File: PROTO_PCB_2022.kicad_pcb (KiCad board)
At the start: 2 copper layers, 92.1 x 40.6 mm, 22 parts, among them J1 HORN_EN1, J10 ECU_KILL_2, J11 ECU_KILL_3, J12 12V_EXTRA, J2 BRAKELIGHTS_EN1, J3 BRAKELIGHTS_CONN, J4 STARTER_MOTOR_EN, J5 VESC_EN_SIGNAL, J6 HORN_CONN, J7 12V_BATT1, J8 ECU_POWER_DIST, J9 ECU_KILL_1, Q1 , Q2 , U1 

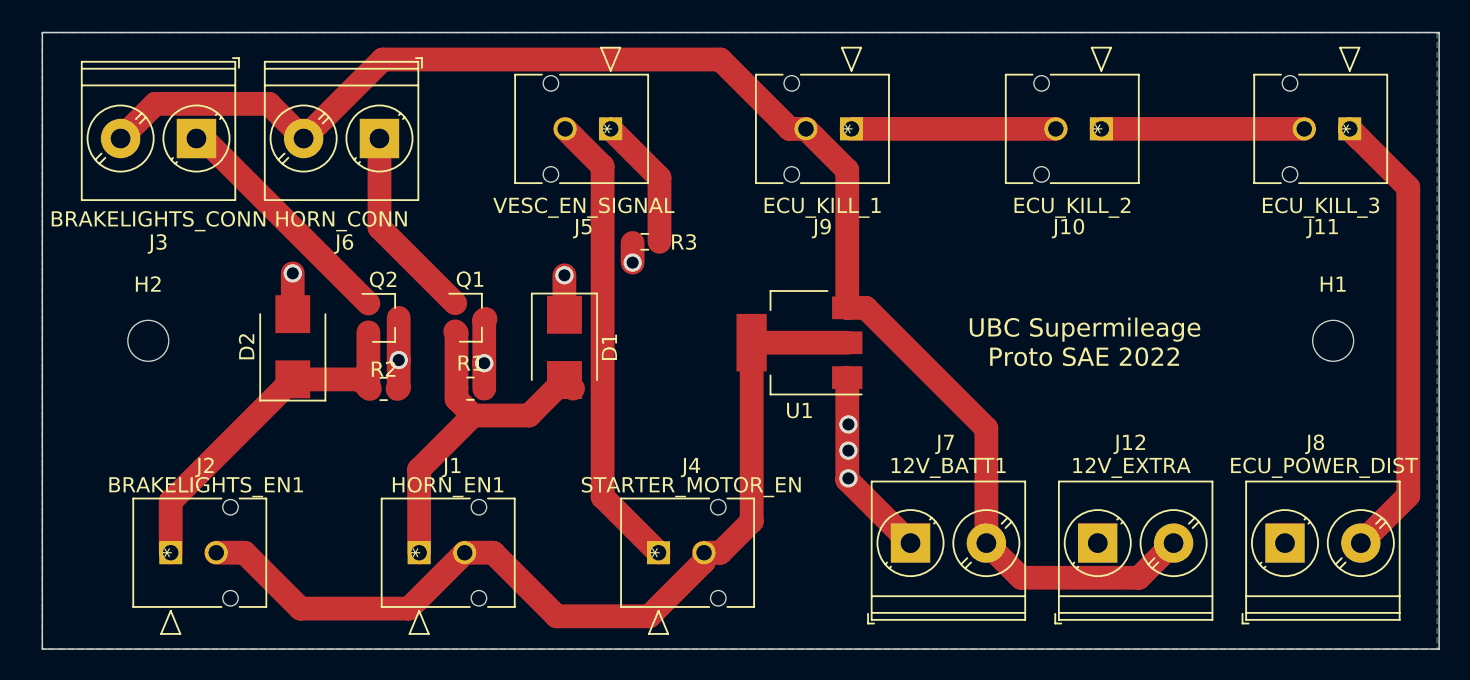
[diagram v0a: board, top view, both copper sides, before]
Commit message: almost final version
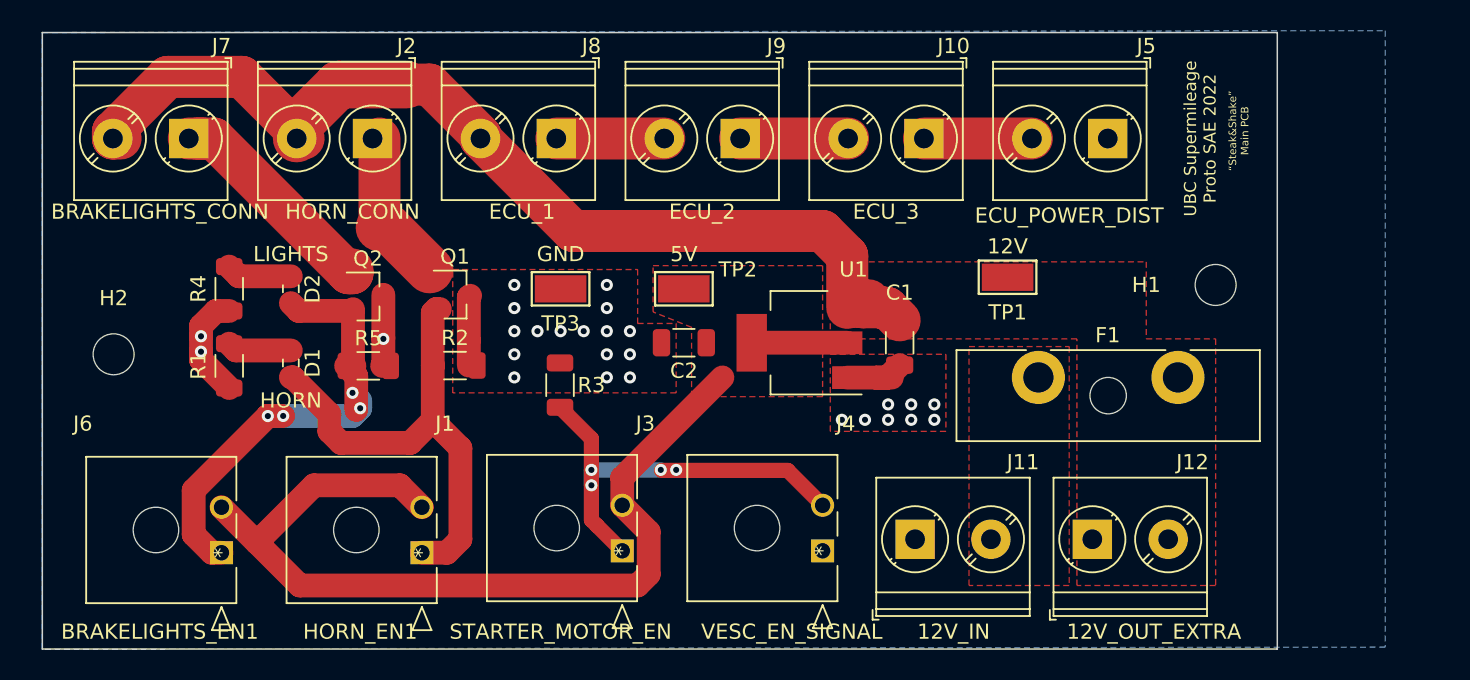
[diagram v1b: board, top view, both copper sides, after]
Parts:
- removed the J11 at (156.7, 84.5)
- added C1: 1u, Capacitor_SMD:C_1206_3216Metric, F.Cu at (127.0, 98.6)
- added C2: 4.7u, Capacitor_SMD:C_1206_3216Metric, F.Cu at (112.8, 98.6)
- added F1: Fuse, Fuse:Fuseholder_Blade_ATO_Littelfuse_Pudenz_2_Pin, F.Cu at (136.1, 100.8)
- added J8: ECU_1, TerminalBlock_Phoenix:TerminalBlock_Phoenix_PT-1,5-2-5.0-H_1x02_P5.00mm_Horizontal, F.Cu at (104.4, 85.1)
- added R1: 4.7k, Resistor_SMD:R_1206_3216Metric, F.Cu at (82.8, 100.1)
- added R4: 4.7k, Resistor_SMD:R_1206_3216Metric, F.Cu at (82.8, 95.0)
- added TP1: TestPoint, TestPoint:TestPoint_Keystone_5015_Micro-Minature, F.Cu at (134.1, 94.2)
- added TP2: TestPoint, TestPoint:TestPoint_Keystone_5015_Micro-Minature, F.Cu at (112.8, 95.0)
- added TP3: TestPoint, TestPoint:TestPoint_Keystone_5015_Micro-Minature, F.Cu at (104.6, 95.0)
- D1, D2: value (none) -> LED; footprint Diode_SMD:D_SMB -> Resistor_SMD:R_0603_1608Metric
- J1: footprint Footprint Library:Molex_Proto_Microfit_Footprint -> footprints:436500201
- J10: value ECU_KILL_2 -> ECU_3; footprint Footprint Library:Molex_Proto_Microfit_Footprint -> TerminalBlock_Phoenix:TerminalBlock_Phoenix_PT-1,5-2-5.0-H_1x02_P5.00mm_Horizontal
- J11: renamed from J7; value 12V_BATT1 -> 12V_IN
- J12: value 12V_EXTRA -> 12V_OUT_EXTRA
- J3: renamed from J4; footprint Footprint Library:Molex_Proto_Microfit_Footprint -> footprints:436500201
- J4: renamed from J5; footprint Footprint Library:Molex_Proto_Microfit_Footprint -> footprints:436500201
- J6: renamed from J2; footprint Footprint Library:Molex_Proto_Microfit_Footprint -> footprints:436500201
- J9: value ECU_KILL_1 -> ECU_2; footprint Footprint Library:Molex_Proto_Microfit_Footprint -> TerminalBlock_Phoenix:TerminalBlock_Phoenix_PT-1,5-2-5.0-H_1x02_P5.00mm_Horizontal
- Q1: value (none) -> HORN_MOSFET1
- Q2: value (none) -> BRAKELIGHTS_MOSFET1
- R2: renamed from R1; footprint Resistor_SMD:R_0805_2012Metric -> Resistor_SMD:R_1206_3216Metric
- R3: value (none) -> 10k; footprint Resistor_SMD:R_0603_1608Metric -> Resistor_SMD:R_1206_3216Metric
- R5: renamed from R2; value (none) -> 10k; footprint Resistor_SMD:R_0805_2012Metric -> Resistor_SMD:R_1206_3216Metric
- U1: value (none) -> LD1117S50TR_SOT223
- moved J4 31.1 mm to (121.9, 112.3), turned to 270 degrees
- moved J5 29.1 mm to (140.7, 85.1), turned to 180 degrees
- moved D1 18.1 mm to (86.9, 99.9)
- moved J10 11.7 mm to (128.6, 85.1), turned to 180 degrees
- moved R3 11.0 mm to (104.6, 101.3), turned to 90 degrees
- moved H1 8.58 mm to (147.8, 94.7)
- moved J9 7.37 mm to (116.5, 85.1), turned to 180 degrees
- moved D2 3.82 mm to (86.9, 95.0), turned to 270 degrees
- moved J6 3.35 mm to (82.3, 112.4)
- moved H2 2.45 mm to (75.2, 99.3)
- moved J3 2.40 mm to (108.7, 112.3)
- moved Q1 1.83 mm to (97.7, 95.4)
- moved R2 1.83 mm to (97.7, 100.1)
- moved R5 1.83 mm to (92.0, 100.1)
- moved Q2 1.75 mm to (91.9, 95.5)
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- renumbered J6 to J2, J8 to J5, J3 to J7
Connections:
- D1 pad 1: GND -> Net-(D1-Pad1)
- D2 pad 1: BRAKELIGHTS_EN_5V -> Net-(D2-Pad1)
- D2 pad 2: GND -> BRAKELIGHTS_EN_5V
- J10 pad 1: ECU_KILL_EN_TOGGLESWITCH_2B -> ECU_KILL_EN_TOGGLESWITCH_3B
- J10 pad 2: ECU_KILL_EN_TOGGLESWITCH_1B -> ECU_KILL_EN_TOGGLESWITCH_2B
- J11 pad 2: 12V_FOR_BRAKELIGHTS -> BATT_12V
- J4 pad 1: Net-(J5-Pad1) -> GND
- J9 pad 1: ECU_KILL_EN_TOGGLESWITCH_1B -> ECU_KILL_EN_TOGGLESWITCH_2B
- J9 pad 2: 12V_FOR_BRAKELIGHTS -> ECU_KILL_EN_TOGGLESWITCH_1B
- R3 pad 1: Net-(J5-Pad1) -> VESC_EN_5V
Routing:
- net 12V_FOR_BRAKELIGHTS: track 98.3 -> 68.5 mm
- net ECU_KILL_EN_TOGGLESWITCH_3B: track 31.2 -> 7.12 mm
- net Net-(J5-Pad1): track 8.78 -> 0.00 mm
- net GND: track 28.6 -> 21.3 mm, vias 8 -> 27
- net HORN_EN_5V: track 24.8 -> 31.6 mm
- net BRAKELIGHTS_EN_5V: track 24.6 -> 31.3 mm, vias 0 -> 4
- net ECU_KILL_EN_TOGGLESWITCH_1B: track 13.5 -> 7.12 mm
- net ECU_KILL_EN_TOGGLESWITCH_2B: track 13.4 -> 7.12 mm
- net +5V: track 61.1 -> 66.4 mm
- net Net-(D2-Pad1): track 0.00 -> 4.33 mm
- net Net-(D1-Pad1): track 0.00 -> 4.25 mm
- net HORN_GND: track 12.9 -> 10.3 mm
- net VESC_EN_5V: track 30.5 -> 28.3 mm, vias 0 -> 4
- net BRAKELIGHTS_GND: track 15.8 -> 15.2 mm
- added copper zone on F.Cu, net +5V
- added copper zone on F.Cu, net 12V_FOR_BRAKELIGHTS
- added copper zone on F.Cu, net BATT_12V
- added copper zone on F.Cu, net GND
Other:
- board size 92.1 x 40.6 mm -> 81.4 x 40.6 mm
- board text added: "12V"
- board text added: "5V"
- board text added: "GND"
- board text added: "HORN"
- board text added: "LIGHTS"
- board text added: "“Steak&Shake” Main PCB"
